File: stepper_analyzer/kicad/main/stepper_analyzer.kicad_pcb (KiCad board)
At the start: 2 copper layers, 81.3 x 66 mm, 37 parts, among them J1 Conn_01x04, J2 Conn_01x04, SW1 SW_Push, SW2 SW_Push, SW3 SW_DIP_x04, U1 ACS70331EESATR-2P5U3, U2 ACS70331EESATR-2P5U3, U3 Teensy 4,0, U4 TFT

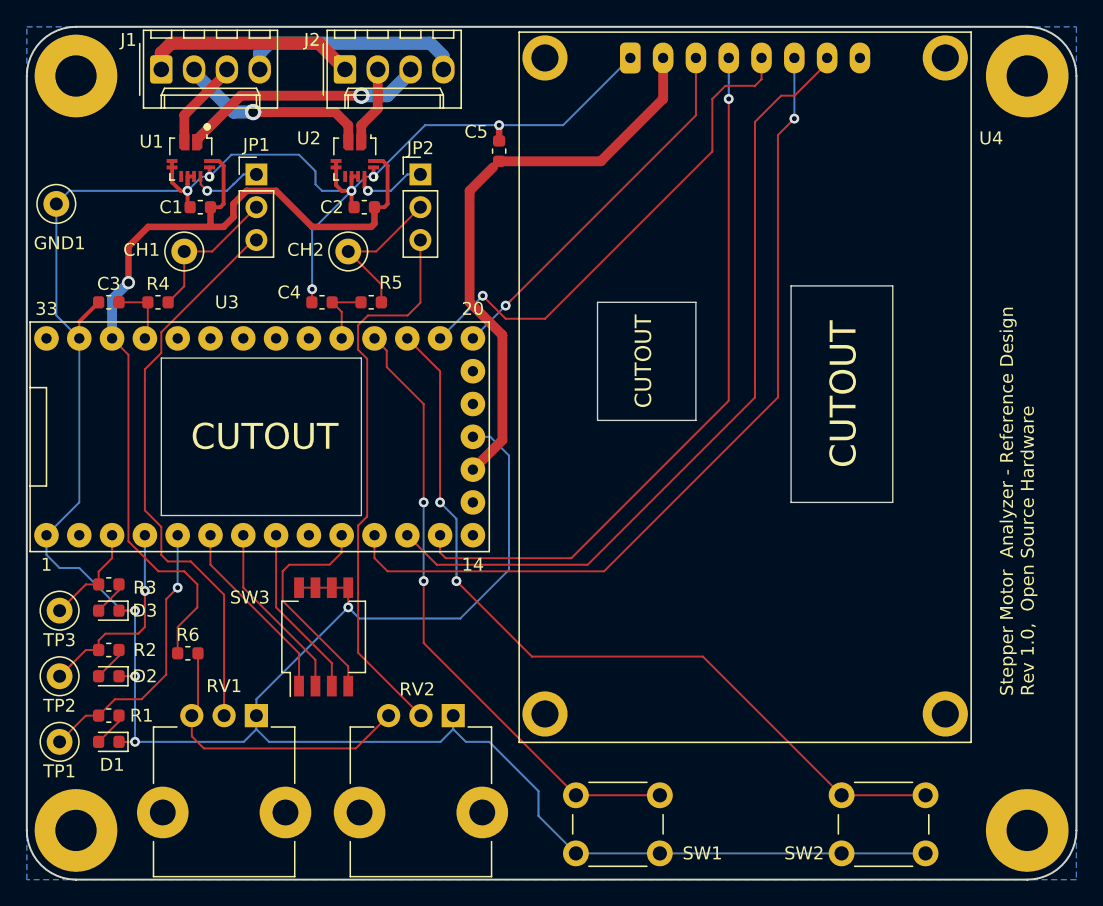
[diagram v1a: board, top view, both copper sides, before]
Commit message: Work in progress.
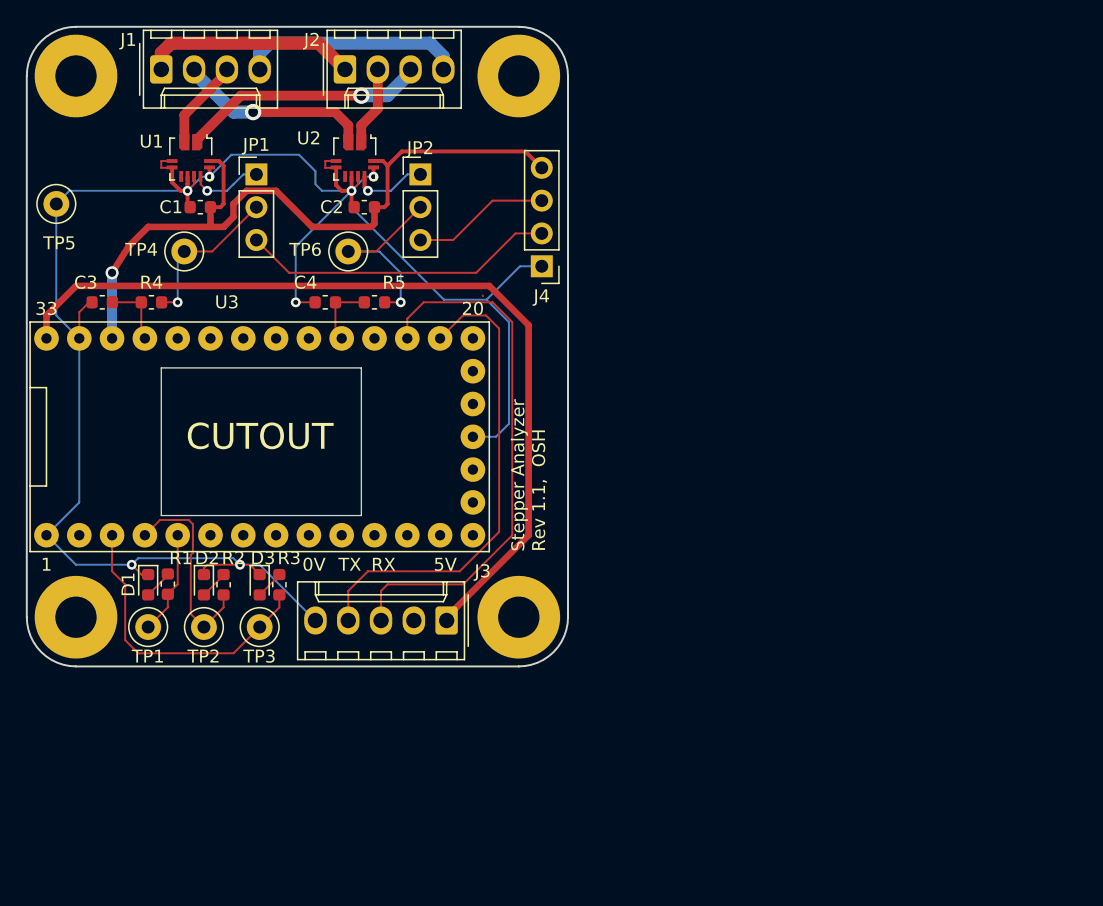
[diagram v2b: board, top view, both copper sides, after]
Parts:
- removed C5: 0.1uF, stepper_analyzer:C_0603_1608Metric
- removed R6: 400R, stepper_analyzer:R_0603_1608Metric
- removed RV1, RV2: 10K, stepper_analyzer:Potentiometer_TT_P0915N
- removed SW1, SW2: SW_Push, stepper_analyzer:SW_PUSH_6mm_H7.3mm
- removed SW3: SW_DIP_x04, stepper_analyzer:SW_DIP_SPSTx04_Slide_Copal_CHS-04B_W7.62mm_P1.27mm
- removed U4: TFT, stepper_analyzer:DIP-TFT
- added J3: Conn_01x05, Connector_Molex:Molex_KK-254_AE-6410-05A_1x05_P2.54mm_Vertical, F.Cu at (144.3, 106.9)
- added J4: Conn_01x04_Female, Connector_PinHeader_2.54mm:PinHeader_1x04_P2.54mm_Vertical, F.Cu at (151.6, 79.5)
- C1, C2: value 0.1uF -> C_Small
- C3, C4: value 0.22uF -> C_Small
- R1, R2, R3: value 3K -> R_Small_US
- R4, R5: value 330R -> R_Small_US
- U1, U2: value ACS70331EESATR-2P5U3 -> ACS70331
- U3: value Teensy 4,0 -> Teensy4-stepper_analyzer
- moved H4 42.7 mm to (149.9, 106.7)
- moved H3 39.4 mm to (149.9, 64.8)
- moved H2 16.5 mm to (115.6, 106.7)
- moved TP3 15.5 mm to (129.8, 107.4)
- moved R3 13.2 mm to (131.3, 104.2), turned to 90 degrees
- moved D1 12.5 mm to (121.2, 104.2), turned to 270 degrees
- moved D3 11.9 mm to (129.8, 104.2), turned to 270 degrees
- moved TP2 11.8 mm to (125.5, 107.4)
- moved TP1 11.2 mm to (121.2, 107.4)
- moved R1 11.2 mm to (122.7, 104.1), turned to 90 degrees
- moved R2 10.2 mm to (127.0, 104.2), turned to 90 degrees
- moved D2 10.2 mm to (125.5, 104.2), turned to 270 degrees
- moved C3 0.51 mm to (117.6, 82.3)
- moved R4 0.51 mm to (121.4, 82.3)
- moved C4 0.25 mm to (134.9, 82.3)
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- renumbered H4 to H2, H2 to H3, H3 to H4, CH1 to TP4, GND1 to TP5, CH2 to TP6
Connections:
- JP1 pad 3: POT1 -> /POT1
- JP2 pad 3: POT2 -> /POT2
- U3 pad 10: Net-(SW3-Pad4) -> (no net)
- U3 pad 11: Net-(U3-Pad11) -> (no net)
- U3 pad 12: Net-(U3-Pad12) -> (no net)
- U3 pad 13: Net-(U3-Pad13) -> (no net)
- U3 pad 16: +3V3D -> (no net)
- U3 pad 20: Net-(U3-Pad20) -> (no net)
- U3 pad 21: Net-(U3-Pad21) -> /SERIAL_OUT
- U3 pad 22: Net-(SW2-Pad2) -> /SERIAL_IN
- U3 pad 23: Net-(SW1-Pad2) -> (no net)
- U3 pad 33: (no net) -> /+5V
- U3 pad 6: Net-(SW3-Pad1) -> (no net)
- U3 pad 7: Net-(SW3-Pad2) -> (no net)
- U3 pad 8: Net-(SW3-Pad3) -> (no net)
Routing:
- net GNDD: track 244.8 -> 154.2 mm, vias 10 -> 7
- net /+5V: track 0.00 -> 66.8 mm
- net Net-(U3-Pad11): track 65.8 -> 0.00 mm, vias 1 -> 0
- net Net-(SW2-Pad2): track 63.6 -> 0.00 mm, vias 2 -> 0
- net Net-(U3-Pad12): track 62.4 -> 0.00 mm
- net Net-(U3-Pad13): track 55.5 -> 0.00 mm, vias 1 -> 0
- net Net-(SW1-Pad2): track 48.3 -> 0.00 mm, vias 2 -> 0
- net +3V3D: track 44.7 -> 0.00 mm
- net POT1: track 44.1 -> 0.00 mm
- net POT2: track 43.2 -> 0.00 mm
- net /SERIAL_IN: track 0.00 -> 41.6 mm
- net Net-(U3-Pad21): track 38.7 -> 0.00 mm, vias 1 -> 0
- net /SERIAL_OUT: track 0.00 -> 37.3 mm
- net Net-(U3-Pad20): track 28.9 -> 0.00 mm, vias 1 -> 0
- net /POT1: track 0.00 -> 24.4 mm
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- removed copper zone on B.Cu, net GNDD
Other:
- board size 81.3 x 66 mm -> 41.9 x 49.5 mm
- board text added: "0V"
- board text added: "5V"
- board text added: "RX"
- board text added: "Stepper Analyzer Rev 1.1, OSH"
- board text added: "TX"
- board text removed: "14"
- board text removed: "CUTOUT"
- board text removed: "Stepper Motor Analyzer - Reference Design Rev 1.0, Open Source Hardware"
